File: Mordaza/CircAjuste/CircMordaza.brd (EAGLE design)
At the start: 125.4 x 74.9 mm, 9 parts, among them IC2 7805TV, X1 SMKDSP_1,5/2

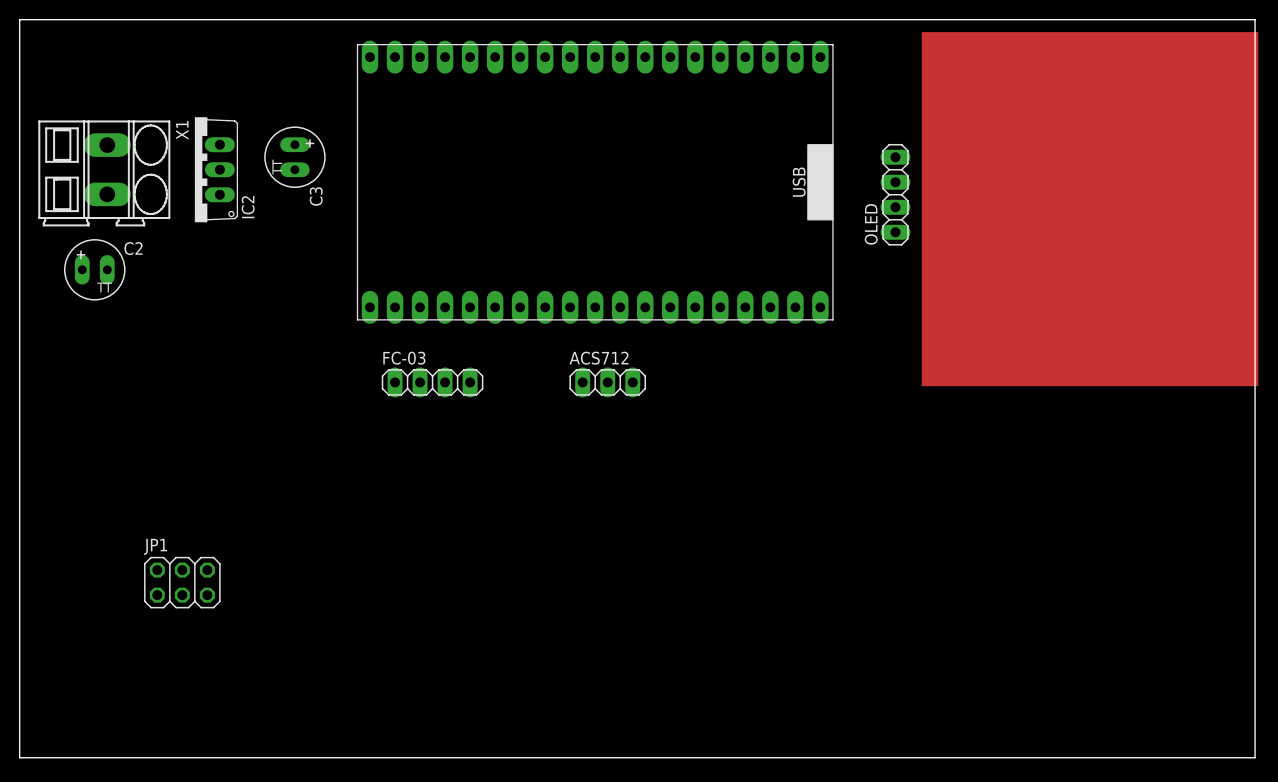
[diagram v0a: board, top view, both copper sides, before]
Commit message: Circuito y prog ok 18/06
Circuito y prog ok 18/06
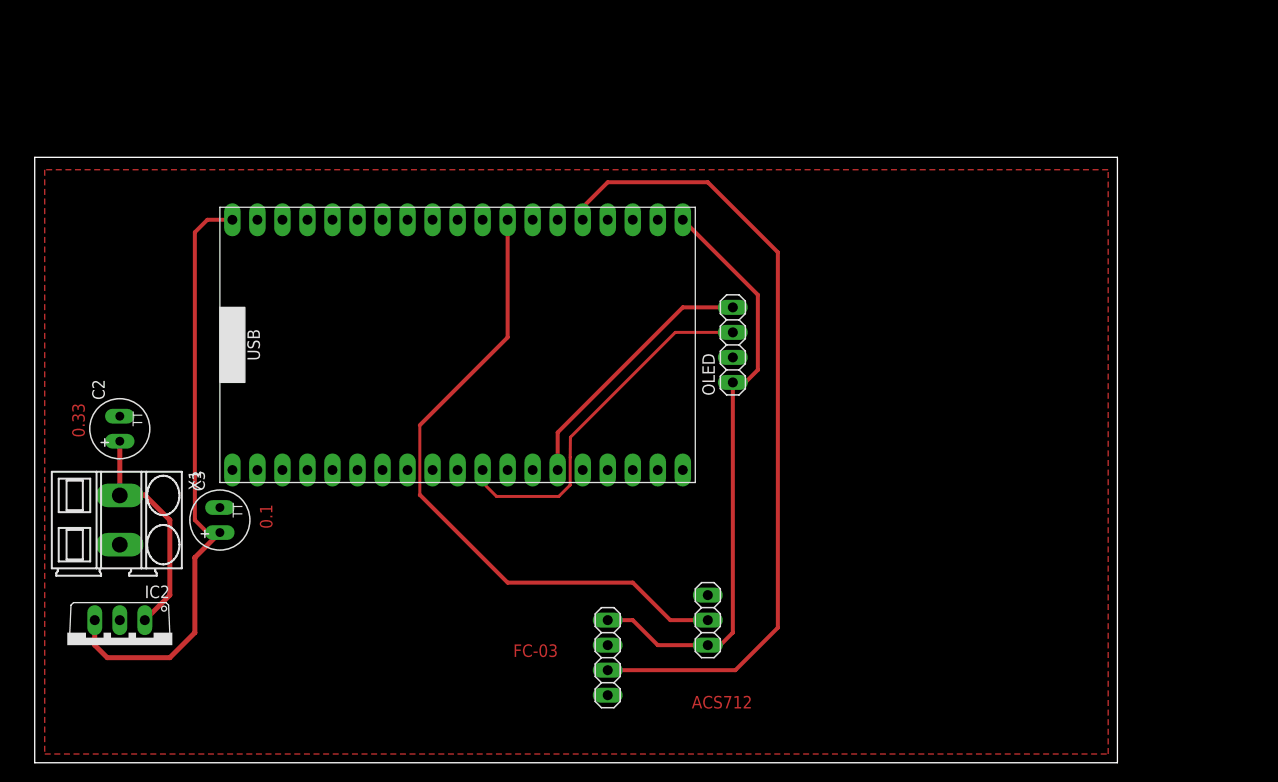
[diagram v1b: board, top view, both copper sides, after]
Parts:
- removed JP1: (no value), pinhead:2X03
- C2: value (none) -> 0.33
- C3: value (none) -> 0.1
- moved U$1 63.3 mm to (20.3, 61.0), turned to 270 degrees
- moved IC2 48.9 mm to (10.2, 16.5), turned to 180 degrees
- moved C3 37.6 mm to (20.3, 29.2), turned to 90 degrees
- moved X1 35.6 mm to (10.2, 29.2)
- moved FC-03 33.1 mm to (59.7, 15.2), turned to 270 degrees
- moved ACS712 26.2 mm to (69.8, 19.1), turned to 90 degrees
- moved OLED 22.5 mm to (72.4, 47.0)
- moved C2 16.3 mm to (10.2, 38.5), turned to 90 degrees
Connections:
- removed net M+: JP1.3
- removed net M-: JP1.4
- removed net SEN+: JP1.5
- removed net SEN-: JP1.6
- removed net VCC_M+: JP1.1
- removed net VCC_M-: JP1.2
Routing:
- net IO34: track 0.00 -> 82.2 mm
- net IO33: track 0.00 -> 66.1 mm
- net +5V: track 0.00 -> 62.1 mm
- net +3V3: track 0.00 -> 61.1 mm
- net SCK: track 0.00 -> 37.0 mm
- net SDA: track 0.00 -> 26.9 mm
- net +12V: track 0.00 -> 22.8 mm
- added copper zone on layer 1, net GND
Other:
- board size 125.4 x 74.9 mm -> 109.9 x 61.5 mm
